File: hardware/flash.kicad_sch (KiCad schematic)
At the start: 14 parts, among them J6 Micro_SD_Card_Det2, U11 W25Q128JVS, U3 ECP5U_12_CABGA256

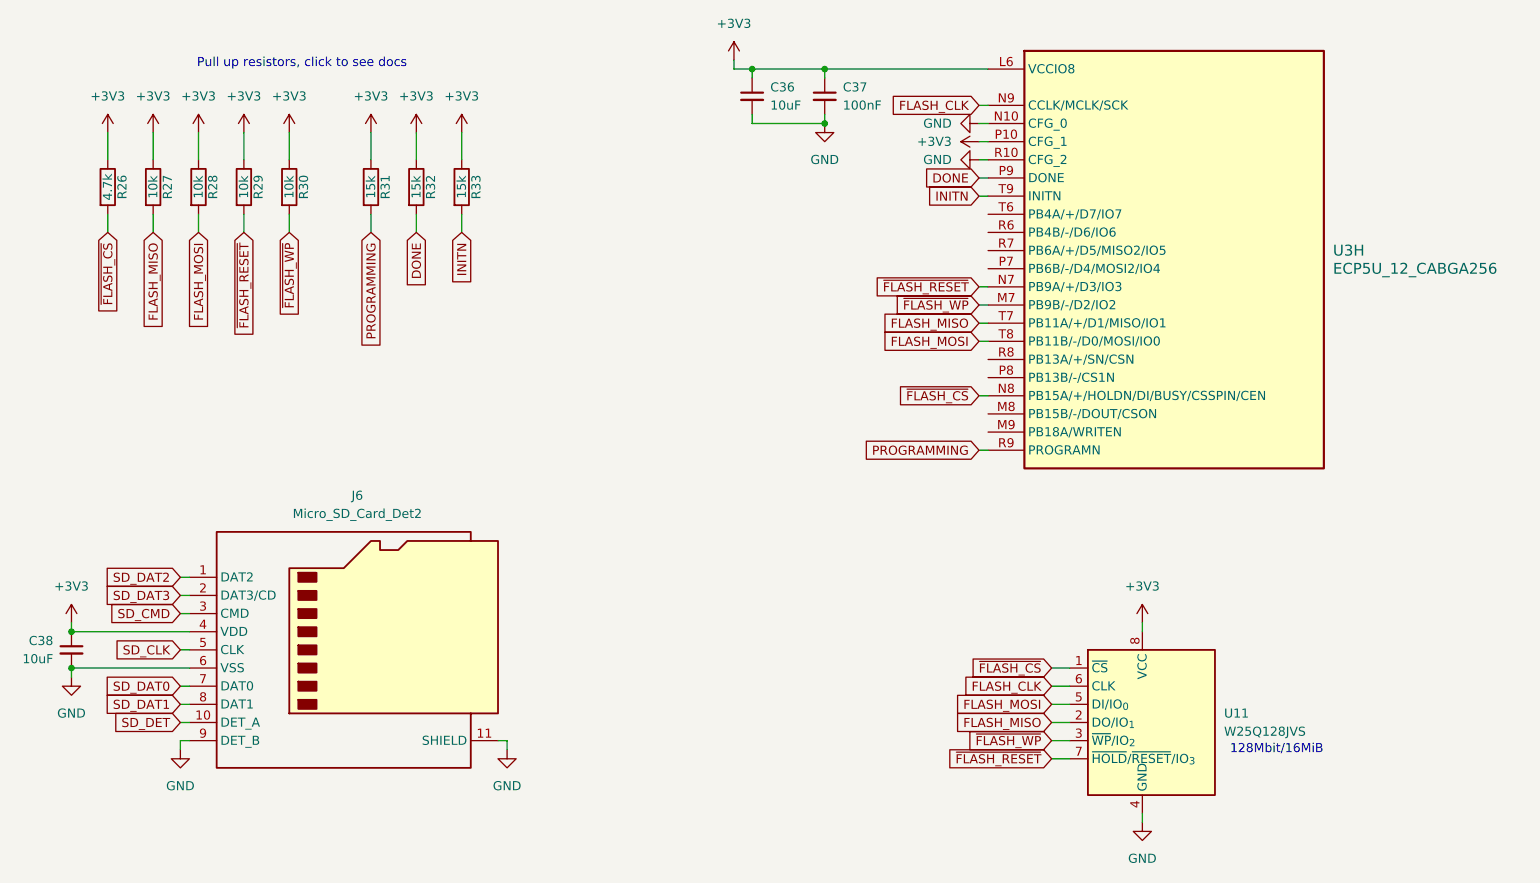
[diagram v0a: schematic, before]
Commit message: Final revision
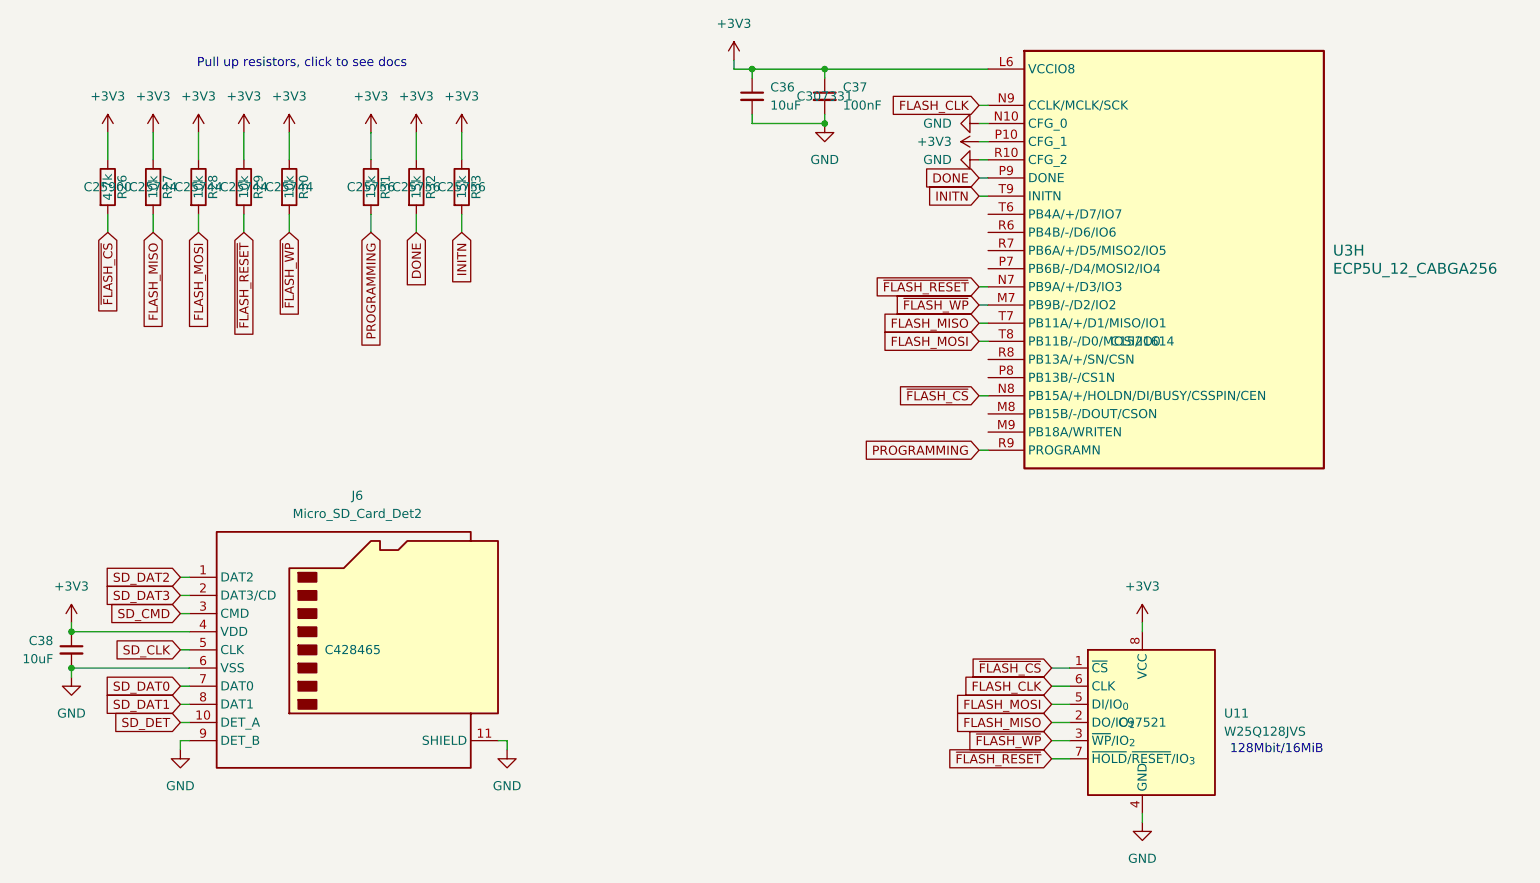
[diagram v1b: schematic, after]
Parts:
- C37: JLCPCB Part # C307331 -> (none); LCSC Part # (none) -> C307331
- J6: JLCPCB Part # C428465 -> (none); LCSC Part # (none) -> C428465
- R26: JLCPCB Part # C25900 -> (none); LCSC Part # (none) -> C25900
- R27, R28, R29, R30: JLCPCB Part # C25744 -> (none); LCSC Part # (none) -> C25744
- R31, R32, R33: JLCPCB Part # C25756 -> (none); LCSC Part # (none) -> C25756
- U11: JLCPCB Part # C97521 -> (none); LCSC Part # (none) -> C97521
- U3: JLCPCB Part # C1521614 -> (none); LCSC Part # (none) -> C1521614
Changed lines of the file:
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@@
 			)
 		)
-		(property "JLCPCB Part #" "C307331 "
+		(property "LCSC Part #" "C307331 "
 			(at 165.1 52.07 0)
 			(effects
@@
 					(size 1.27 1.27)
 				)
-				(hide yes)
 			)
 		)
@@
 			)
 		)
-		(property "JLCPCB Part #" "C97521"
+		(property "LCSC Part #" "C97521"
 			(at 209.55 139.7 0)
 			(effects
@@
 					(size 1.27 1.27)
 				)
-				(hide yes)
 			)
 		)
@@
 			)
 		)
-		(property "JLCPCB Part #" "C25756 "
+		(property "LCSC Part #" "C25756 "
 			(at 101.6 64.77 0)
 			(effects
@@
 					(size 1.27 1.27)
 				)
-				(hide yes)
 			)
 		)
@@
 			)
 		)
-		(property "JLCPCB Part #" "C25756 "
+		(property "LCSC Part #" "C25756 "
 			(at 107.95 64.77 0)
 			(effects
@@
 					(size 1.27 1.27)
 				)
-				(hide yes)
 			)
 		)
@@
 			)
 		)
-		(property "JLCPCB Part #" "C1521614"
+		(property "LCSC Part #" "C1521614"
 			(at 209.55 86.36 0)
 			(effects
@@
 					(size 1.27 1.27)
 				)
-				(hide yes)
 			)
 		)
@@
 			)
 		)
-		(property "JLCPCB Part #" "C25744"
+		(property "LCSC Part #" "C25744"
 			(at 83.82 64.77 0)
 			(effects
@@
 					(size 1.27 1.27)
 				)
-				(hide yes)
 			)
 		)
@@
 			)
 		)
-		(property "JLCPCB Part #" "C25756 "
+		(property "LCSC Part #" "C25756 "
 			(at 114.3 64.77 0)
 			(effects
@@
 					(size 1.27 1.27)
 				)
-				(hide yes)
 			)
 		)
@@
 			)
 		)
-		(property "JLCPCB Part #" "C25900 "
+		(property "LCSC Part #" "C25900 "
 			(at 64.77 64.77 0)
 			(effects
@@
 					(size 1.27 1.27)
 				)
-				(hide yes)
 			)
 		)
@@
 			)
 		)
-		(property "JLCPCB Part #" "C25744"
+		(property "LCSC Part #" "C25744"
 			(at 71.12 64.77 0)
 			(effects
@@
 					(size 1.27 1.27)
 				)
-				(hide yes)
 			)
 		)
@@
 			)
 		)
-		(property "JLCPCB Part #" "C25744"
+		(property "LCSC Part #" "C25744"
 			(at 90.17 64.77 0)
 			(effects
@@
 					(size 1.27 1.27)
 				)
-				(hide yes)
 			)
 		)
@@
 			)
 		)
-		(property "JLCPCB Part #" "C428465"
+		(property "LCSC Part #" "C428465"
 			(at 99.06 129.54 0)
 			(effects
@@
 					(size 1.27 1.27)
 				)
-				(hide yes)
 			)
 		)
@@
 			)
 		)
-		(property "JLCPCB Part #" "C25744"
+		(property "LCSC Part #" "C25744"
 			(at 77.47 64.77 0)
 			(effects
@@
 					(size 1.27 1.27)
 				)
-				(hide yes)
-			)
-		)
+			)
+		)

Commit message: Last checks
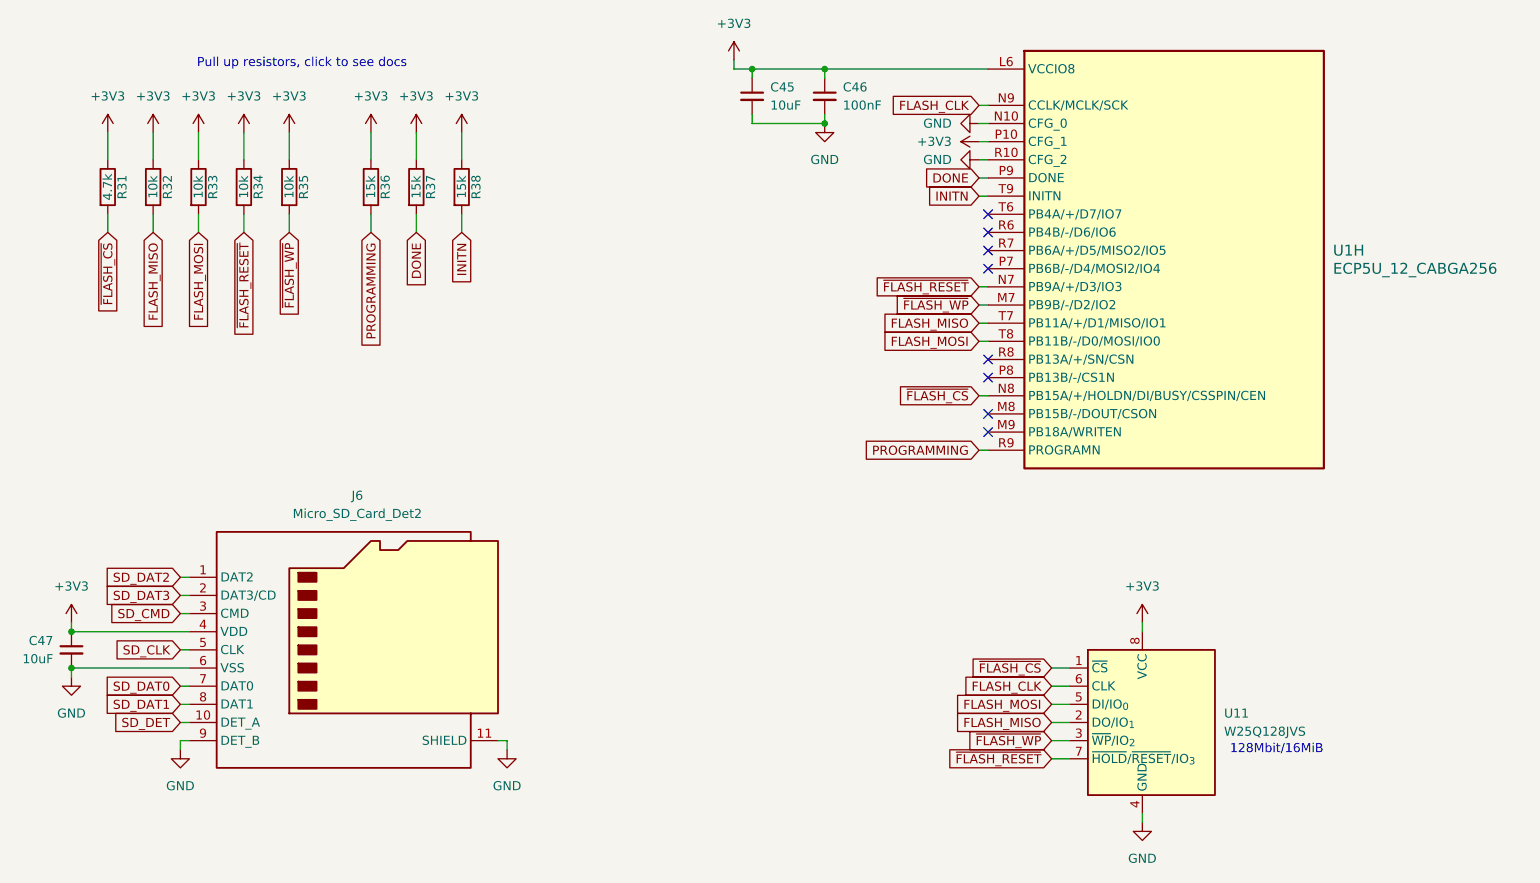
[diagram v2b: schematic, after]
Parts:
- C45: renamed from C36; LCSC Part # (none) -> C19702
- C47: renamed from C38; LCSC Part # (none) -> C19702
- renumbered C37 to C46, R26 to R31, R27 to R32, R28 to R33, R29 to R34, R30 to R35, R31 to R36, R32 to R37, R33 to R38, U3 to U1
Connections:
- no-connect marks 0 -> 8
